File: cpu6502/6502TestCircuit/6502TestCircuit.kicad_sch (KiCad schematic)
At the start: 15 parts, among them J1 Power, J2 Power, J3 Reset, SW1 Reset, U6 L7805, U9 DS1813

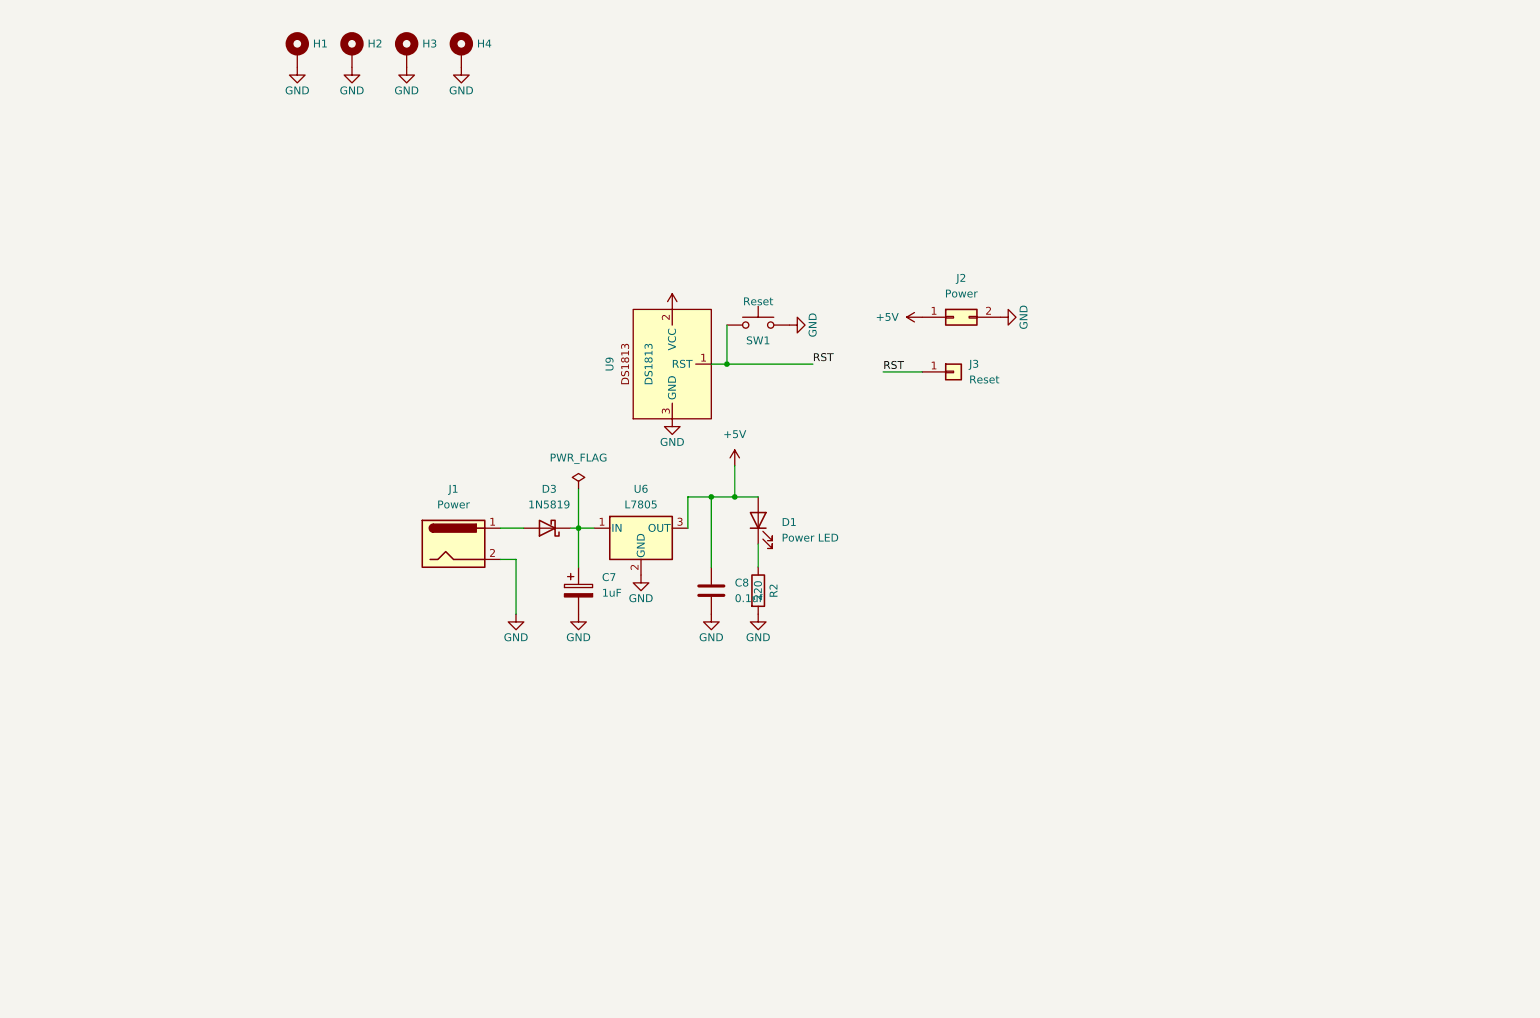
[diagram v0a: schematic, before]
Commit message: code changes (wip), set test PCB 2.0 to PCBway
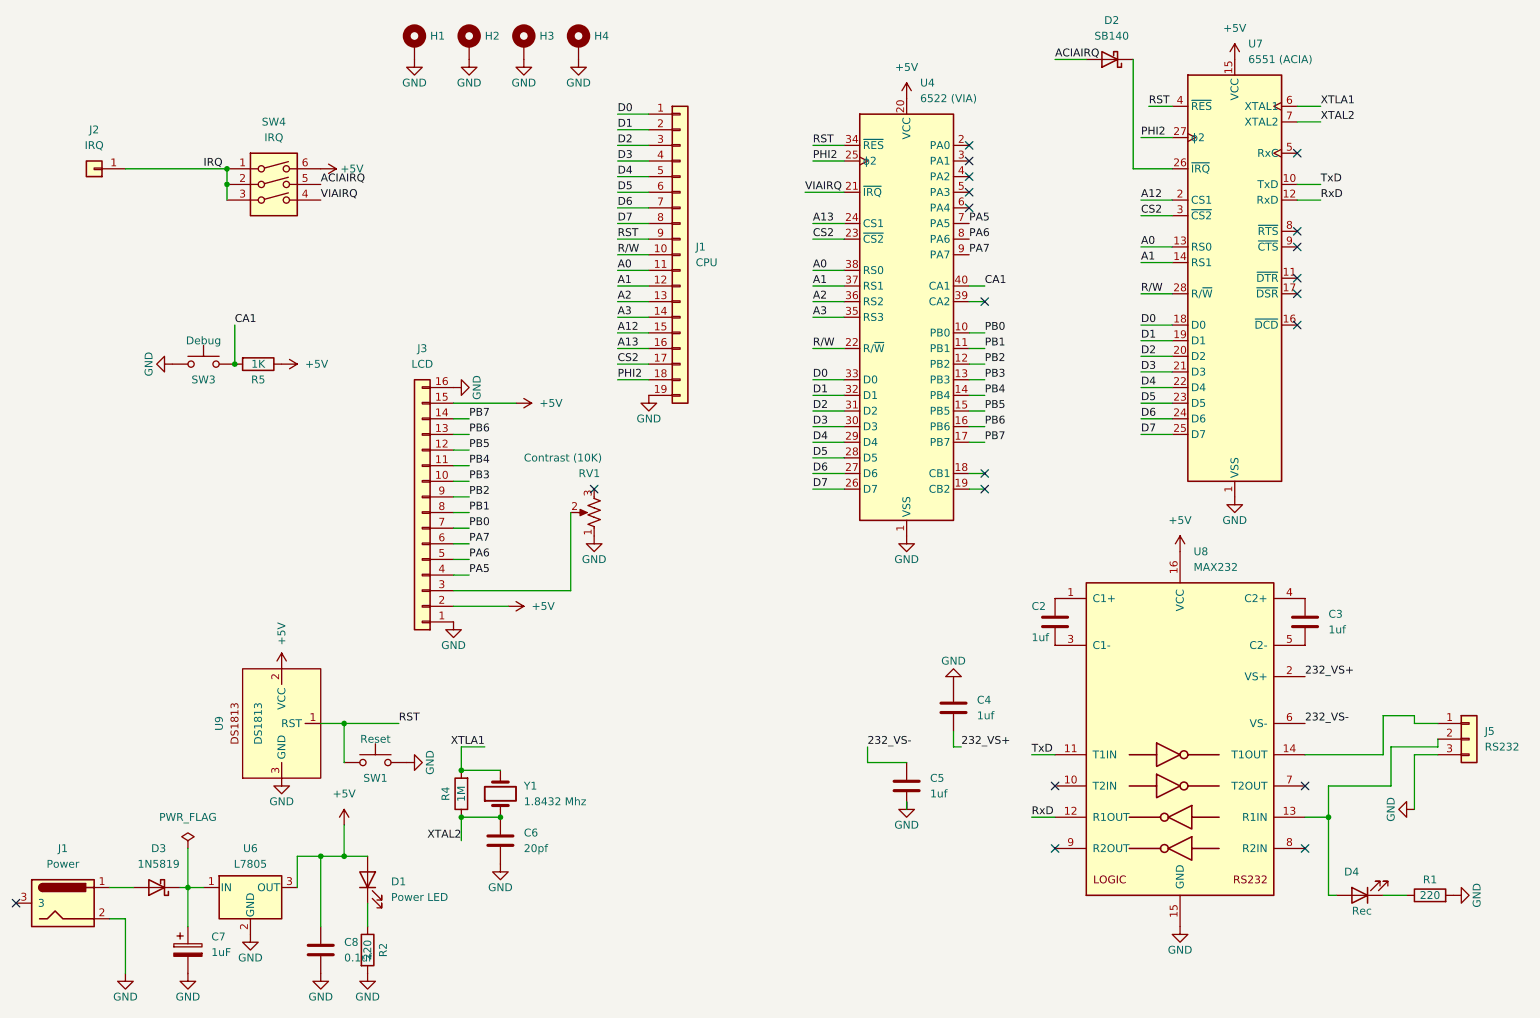
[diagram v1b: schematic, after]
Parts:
- removed J2: Power, Connector_PinHeader_2.54mm:PinHeader_2x01_P2.54mm_Vertical, symbol Connector_Generic:Conn_02x01
- removed J3: Reset, Connector_PinHeader_2.54mm:PinHeader_1x01_P2.54mm_Vertical, symbol Connector_Generic:Conn_01x01
- added C2, C3, C4, C5: 1uf, Capacitor_THT:C_Disc_D3.0mm_W1.6mm_P2.50mm, symbol Device:C
- added C6: 20pf, Capacitor_THT:C_Disc_D3.0mm_W1.6mm_P2.50mm, symbol Device:C
- added D2: SB140, Diode_THT:D_DO-41_SOD81_P10.16mm_Horizontal, symbol Diode:SB140
- added D4: Rec, LED_THT:LED_D3.0mm, symbol Device:LED
- added J1: CPU, Connector_PinHeader_2.54mm:PinHeader_1x19_P2.54mm_Vertical, symbol Connector_Generic:Conn_01x19
- added J2: IRQ, Connector_PinHeader_2.54mm:PinHeader_1x01_P2.54mm_Vertical, symbol Connector_Generic:Conn_01x01
- added J3: LCD, Connector_PinHeader_2.54mm:PinHeader_1x16_P2.54mm_Vertical, symbol Connector_Generic:Conn_01x16
- added J5: RS232, TerminalBlock_TE-Connectivity:TerminalBlock_TE_282834-3_1x03_P2.54mm_Horizontal, symbol Connector_Generic:Conn_01x03
- added R1: 220, Resistor_THT:R_Axial_DIN0207_L6.3mm_D2.5mm_P2.54mm_Vertical, symbol Device:R
- added R4: 1M, Resistor_THT:R_Axial_DIN0204_L3.6mm_D1.6mm_P7.62mm_Horizontal, symbol Device:R
- added R5: 1K, Resistor_THT:R_Axial_DIN0204_L3.6mm_D1.6mm_P2.54mm_Vertical, symbol Device:R
- added RV1: Contrast (10K), Potentiometer_THT:Potentiometer_Bourns_3386P_Vertical, symbol Device:R_Potentiometer_US
- added SW3: Debug, Button_Switch_THT:SW_TH_Tactile_Omron_B3F-10xx, symbol Switch:SW_Push
- added SW4: IRQ, Button_Switch_THT:SW_DIP_SPSTx03_Slide_6.7x9.18mm_W7.62mm_P2.54mm_LowProfile, symbol Switch:SW_DIP_x03
- added U4: 6522 (VIA), Package_DIP:DIP-40_W15.24mm_Socket, symbol PCM_65xx-library:W65C22NxP
- added U7: 6551 (ACIA), Package_DIP:DIP-28_W15.24mm_Socket, symbol PCM_65xx-library:W65C51NxP
- added U8: MAX232, Package_DIP:DIP-16_W7.62mm_Socket, symbol Interface_UART:MAX232
- added Y1: 1.8432 Mhz, Crystal:Crystal_HC49-4H_Vertical, symbol Device:Crystal
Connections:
- net +5V: now also J3.15 (Pin_15), J3.2 (Pin_2), R5.1, SW4.6, U4.20 (VCC), U7.15 (VCC), U8.16 (VCC)
- net GND: now also C4.1, C5.2, C6.2, J1.19 (Pin_19), J3.1 (Pin_1), J3.16 (Pin_16), J5.3 (Pin_3), R1.2, RV1.1, SW3.1, U4.1 (VSS), U7.1 (VSS), U8.15 (GND)
- net RST: now also J1.9 (Pin_9), U4.34 (~{RES}), U7.4 (~{RES})
- new net: D4.1 (K), R1.1
- new net: D2.1 (K), U7.26 (~{IRQ})
- new net: J3.3 (Pin_3), RV1.2
- new net: J5.1 (Pin_1), U8.14 (T1OUT)
- new net: D4.2 (A), J5.2 (Pin_2), U8.13 (R1IN)
- new net: C2.1, U8.1 (C1+)
- new net: C2.2, U8.3 (C1-)
- new net: C3.1, U8.4 (C2+)
- new net: C3.2, U8.5 (C2-)
- new net 232_VS+: C4.2, U8.2 (VS+)
- new net 232_VS-: C5.1, U8.6 (VS-)
- new net A0: J1.11 (Pin_11), U4.38 (RS0), U7.13 (RS0)
- new net A1: J1.12 (Pin_12), U4.37 (RS1), U7.14 (RS1)
- new net A12: J1.15 (Pin_15), U7.2 (CS1)
- new net A13: J1.16 (Pin_16), U4.24 (CS1)
- new net A2: J1.13 (Pin_13), U4.36 (RS2)
- new net A3: J1.14 (Pin_14), U4.35 (RS3)
- new net ACIAIRQ: D2.2 (A), SW4.5
- new net CA1: R5.2, SW3.2, U4.40 (CA1)
- new net CS2: J1.17 (Pin_17), U4.23 (~{CS2}), U7.3 (~{CS2})
- new net D0: J1.1 (Pin_1), U4.33 (D0), U7.18 (D0)
- new net D1: J1.2 (Pin_2), U4.32 (D1), U7.19 (D1)
- new net D2: J1.3 (Pin_3), U4.31 (D2), U7.20 (D2)
- new net D3: J1.4 (Pin_4), U4.30 (D3), U7.21 (D3)
- new net D4: J1.5 (Pin_5), U4.29 (D4), U7.22 (D4)
- new net D5: J1.6 (Pin_6), U4.28 (D5), U7.23 (D5)
- new net D6: J1.7 (Pin_7), U4.27 (D6), U7.24 (D6)
- new net D7: J1.8 (Pin_8), U4.26 (D7), U7.25 (D7)
- new net IRQ: J2.1 (Pin_1), SW4.1, SW4.2, SW4.3
- new net PA5: J3.4 (Pin_4), U4.7 (PA5)
- new net PA6: J3.5 (Pin_5), U4.8 (PA6)
- new net PA7: J3.6 (Pin_6), U4.9 (PA7)
- new net PB0: J3.7 (Pin_7), U4.10 (PB0)
- new net PB1: J3.8 (Pin_8), U4.11 (PB1)
- new net PB2: J3.9 (Pin_9), U4.12 (PB2)
- new net PB3: J3.10 (Pin_10), U4.13 (PB3)
- new net PB4: J3.11 (Pin_11), U4.14 (PB4)
- new net PB5: J3.12 (Pin_12), U4.15 (PB5)
- new net PB6: J3.13 (Pin_13), U4.16 (PB6)
- new net PB7: J3.14 (Pin_14), U4.17 (PB7)
- new net PHI2: J1.18 (Pin_18), U4.25 (ϕ2), U7.27 (ϕ2)
- new net RxD: U7.12 (RxD), U8.12 (R1OUT)
- new net R/W: J1.10 (Pin_10), U4.22 (R/~{W}), U7.28 (R/~{W})
- new net TxD: U7.10 (TxD), U8.11 (T1IN)
- new net VIAIRQ: SW4.4, U4.21 (~{IRQ})
- new net XTAL2: C6.1, R4.1, U7.7 (XTAL2), Y1.1
- new net XTLA1: R4.2, U7.6 (XTAL1), Y1.2
- no-connect marks 0 -> 20
